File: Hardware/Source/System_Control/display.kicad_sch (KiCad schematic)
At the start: 9 parts, among them Q3 MMBT2222A, U5 LCD 5“SSD1963

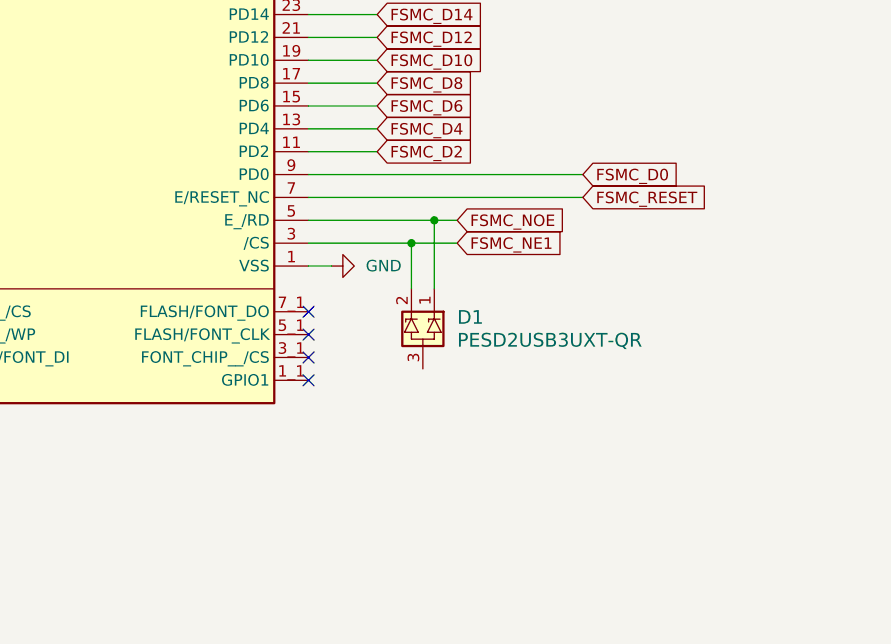
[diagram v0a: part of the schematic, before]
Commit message: update
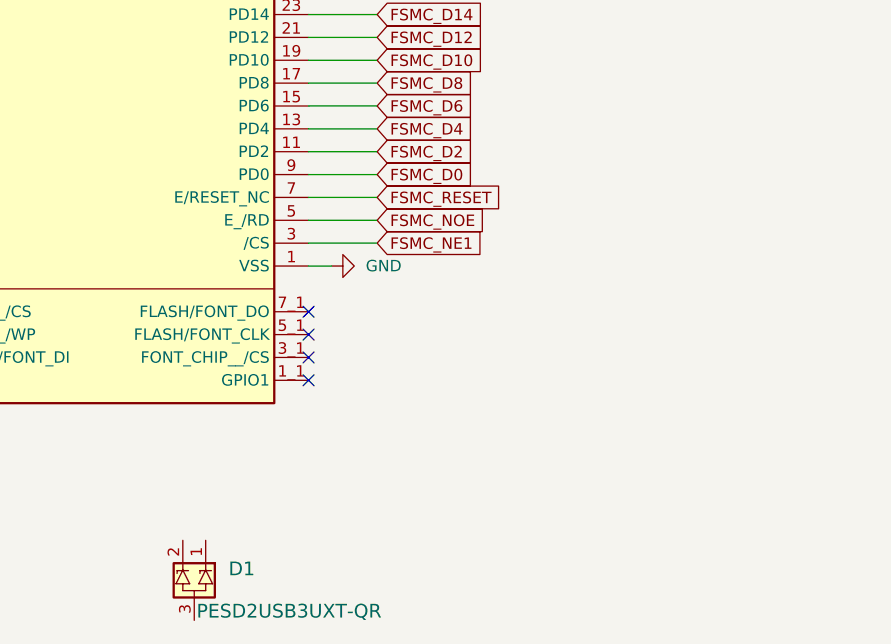
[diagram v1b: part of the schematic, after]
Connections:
- net FSMC_NE1: no longer D1.2
- net FSMC_NOE: no longer D1.1
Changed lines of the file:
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@@
 	(paper "A4")
-	(junction
-		(at 181.61 99.06)
-		(diameter 0)
-		(color 0 0 0 0)
-	)
 	(junction
 		(at 78.74 55.88)
@@
 	)
 	(junction
-		(at 179.07 101.6)
-		(diameter 0)
-		(color 0 0 0 0)
-	)
-	(junction
 		(at 241.3 100.33)
 		(diameter 0)
@@
 	(wire
 		(pts
-			(xy 179.07 101.6) (xy 167.64 101.6)
+			(xy 167.64 101.6) (xy 175.26 101.6)
 		)
 		(stroke
@@
 	(wire
 		(pts
-			(xy 184.15 99.06) (xy 181.61 99.06)
-		)
-		(stroke
-			(width 0)
-			(type default)
-		)
-	)
-	(wire
-		(pts
 			(xy 78.74 40.64) (xy 78.74 44.45)
 		)
@@
 	(wire
 		(pts
-			(xy 179.07 101.6) (xy 184.15 101.6)
-		)
-		(stroke
-			(width 0)
-			(type default)
-		)
-	)
-	(wire
-		(pts
 			(xy 115.57 63.5) (xy 123.19 63.5)
 		)
@@
 	(wire
 		(pts
-			(xy 198.12 93.98) (xy 167.64 93.98)
+			(xy 175.26 93.98) (xy 167.64 93.98)
 		)
 		(stroke
@@
 	(wire
 		(pts
-			(xy 167.64 96.52) (xy 198.12 96.52)
+			(xy 167.64 96.52) (xy 175.26 96.52)
 		)
 		(stroke
@@
 	(wire
 		(pts
-			(xy 181.61 99.06) (xy 167.64 99.06)
+			(xy 167.64 99.06) (xy 175.26 99.06)
 		)
 		(stroke
@@
 	(wire
 		(pts
-			(xy 179.07 101.6) (xy 179.07 106.68)
-		)
-		(stroke
-			(width 0)
-			(type default)
-		)
-	)
-	(wire
-		(pts
 			(xy 115.57 55.88) (xy 123.19 55.88)
 		)
@@
 		(pts
 			(xy 78.74 57.15) (xy 78.74 55.88)
-		)
-		(stroke
-			(width 0)
-			(type default)
-		)
-	)
-	(wire
-		(pts
-			(xy 181.61 99.06) (xy 181.61 106.68)
 		)
 		(stroke
@@
 	(global_label "FSMC_NE1"
 		(shape input)
-		(at 184.15 101.6 0)
+		(at 175.26 101.6 0)
 		(fields_autoplaced yes)
 		(effects
@@
 		)
 		(property "Intersheetrefs" "${INTERSHEET_REFS}"
-			(at 196.8113 101.6 0)
+			(at 187.9213 101.6 0)
 			(effects
 				(font
@@
 	(global_label "FSMC_NOE"
 		(shape input)
-		(at 184.15 99.06 0)
+		(at 175.26 99.06 0)
 		(fields_autoplaced yes)
 		(effects
@@
 		)
 		(property "Intersheetrefs" "${INTERSHEET_REFS}"
-			(at 196.9323 99.06 0)
+			(at 188.0423 99.06 0)
 			(effects
 				(font
@@
 	(global_label "FSMC_RESET"
 		(shape input)
-		(at 198.12 96.52 0)
+		(at 175.26 96.52 0)
 		(fields_autoplaced yes)
 		(effects
@@
 		)
 		(property "Intersheetrefs" "${INTERSHEET_REFS}"
-			(at 212.8374 96.52 0)
+			(at 189.9774 96.52 0)
 			(effects
 				(font
@@
 	(global_label "FSMC_D0"
 		(shape input)
-		(at 198.12 93.98 0)
+		(at 175.26 93.98 0)
 		(fields_autoplaced yes)
 		(effects
@@
 		)
 		(property "Intersheetrefs" "${INTERSHEET_REFS}"
-			(at 209.5718 93.98 0)
+			(at 186.7118 93.98 0)
 			(effects
 				(font
@@
 	)
 	(symbol
-		(lib_id "charge_battery_sym_lib:PESD2USB3UXT-QR")
-		(at 177.8 109.22 270)
-		(unit 1)
-		(exclude_from_sim no)
-		(in_bom yes)
-		(on_board yes)
-		(dnp no)
-		(fields_autoplaced yes)
-		(property "Reference" "D1"
-			(at 184.15 109.8549 90)
-			(effects
-				(font
-					(size 1.524 1.524)
-				)
-				(justify left)
-			)
-		)
-		(property "Value" "PESD2USB3UXT-QR"
-			(at 184.15 112.3949 90)
-			(effects
-				(font
-					(size 1.524 1.524)
-				)
-				(justify left)
-			)
-		)
-		(property "Footprint" "charge_battery_footprint_lib:SOT23"
-			(at 165.608 113.792 0)
-			(effects
-				(font
-					(size 1.27 1.27)
-					(italic yes)
-				)
-				(hide yes)
-			)
-		)
-		(property "Datasheet" "https://www.mouser.vn/datasheet/2/916/PESD2USB3UXT_Q-3435971.pdf"
-			(at 165.608 114.808 0)
-			(effects
-				(font
-					(size 1.27 1.27)
-					(italic yes)
-				)
-				(hide yes)
-			)
-		)
-		(property "Description" "ESD Protection Diodes / TVS Diodes SOT23 3.3V 4A AUTO ESD PROT"
-			(at 165.608 109.982 0)
-			(effects
-				(font
-					(size 1.27 1.27)
-				)
-				(hide yes)
-			)
-		)
-		(property "Supply name" "Mouser"
-			(at 165.608 110.49 0)
-			(effects
-				(font
-					(size 1.27 1.27)
-				)
-				(hide yes)
-			)
-		)
-		(property "Supply part number" "771-PESD2USB3UXT-QR"
-			(at 165.608 110.744 0)
-			(effects
-				(font
-					(size 1.27 1.27)
-				)
-				(hide yes)
-			)
-		)
-		(property "Supply URL" "https://www.mouser.vn/ProductDetail/Nexperia/PESD2USB3UXT-QR?qs=3Rah4i%252BhyCErbBl4ep9%252BDw%3D%3D"
-			(at 165.608 110.744 0)
-			(effects
-				(font
-					(size 1.27 1.27)
-				)
-				(hide yes)
-			)
-		)
-		(pin "3"
-		)
-		(pin "1"
-		)
-		(pin "2"
-		)
-		(instances
-			(project ""
-				(path "/85c53e8c-0403-413d-b6c5-0718d4365b1f/acaf0f73-9448-4a46-8e0c-1a18f2f42e7d"
-					(reference "D1")
-					(unit 1)
-				)
-			)
-		)
-	)
-	(symbol
 		(lib_id "charge_battery_sym_lib:Res_1K_0603_1%")
 		(at 39.37 62.23 0)
@@
 					(unit 1)
 				)
+			)
+		)
+	)
+	(symbol
+		(lib_id "charge_battery_sym_lib:PESD2USB3UXT-QR")
+		(at 152.4 137.16 270)
+		(unit 1)
+		(exclude_from_sim no)
+		(in_bom yes)
+		(on_board yes)
+		(dnp no)
+		(property "Reference" "D1"
+			(at 158.75 137.7949 90)
+			(effects
+				(font
+					(size 1.524 1.524)
+				)
+				(justify left)
+			)
+		)
+		(property "Value" "PESD2USB3UXT-QR"
+			(at 155.194 142.494 90)
+			(effects
+				(font
+					(size 1.524 1.524)
+				)
+				(justify left)
+			)
+		)
+		(property "Footprint" "charge_battery_footprint_lib:SOT23"
+			(at 140.208 141.732 0)
+			(effects
+				(font
+					(size 1.27 1.27)
+					(italic yes)
+				)
+				(hide yes)
+			)
+		)
+		(property "Datasheet" "https://www.mouser.vn/datasheet/2/916/PESD2USB3UXT_Q-3435971.pdf"
+			(at 140.208 142.748 0)
+			(effects
+				(font
+					(size 1.27 1.27)
+					(italic yes)
+				)
+				(hide yes)
+			)
+		)
+		(property "Description" "ESD Protection Diodes / TVS Diodes SOT23 3.3V 4A AUTO ESD PROT"
+			(at 140.208 137.922 0)
+			(effects
+				(font
+					(size 1.27 1.27)
+				)
+				(hide yes)
+			)
+		)
+		(property "Supply name" "Mouser"
+			(at 140.208 138.43 0)
+			(effects
+				(font
+					(size 1.27 1.27)
+				)
+				(hide yes)
+			)
+		)
+		(property "Supply part number" "771-PESD2USB3UXT-QR"
+			(at 140.208 138.684 0)
+			(effects
+				(font
+					(size 1.27 1.27)
+				)
+				(hide yes)
+			)
+		)
+		(property "Supply URL" "https://www.mouser.vn/ProductDetail/Nexperia/PESD2USB3UXT-QR?qs=3Rah4i%252BhyCErbBl4ep9%252BDw%3D%3D"
+			(at 140.208 138.684 0)
+			(effects
+				(font
+					(size 1.27 1.27)
+				)
+				(hide yes)
+			)
+		)
+		(pin "3"
+		)
+		(pin "1"
+		)
+		(pin "2"
+		)
+		(instances
+			(project "System_Control"
+				(path "/85c53e8c-0403-413d-b6c5-0718d4365b1f/acaf0f73-9448-4a46-8e0c-1a18f2f42e7d"
+					(reference "D1")
+					(unit 1)
+				)

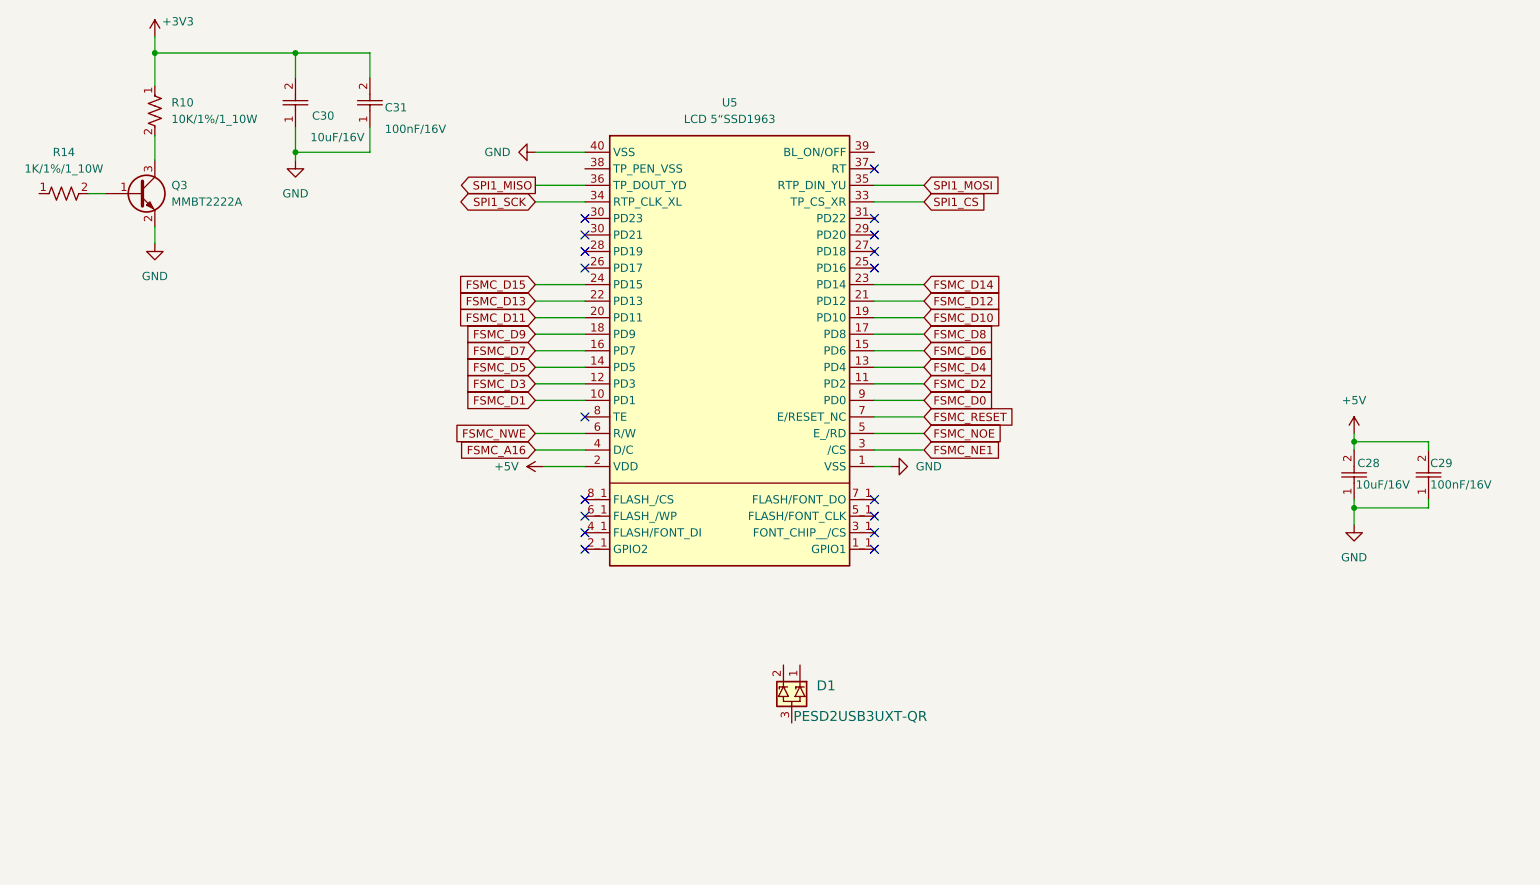
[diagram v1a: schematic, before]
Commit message: update footprint
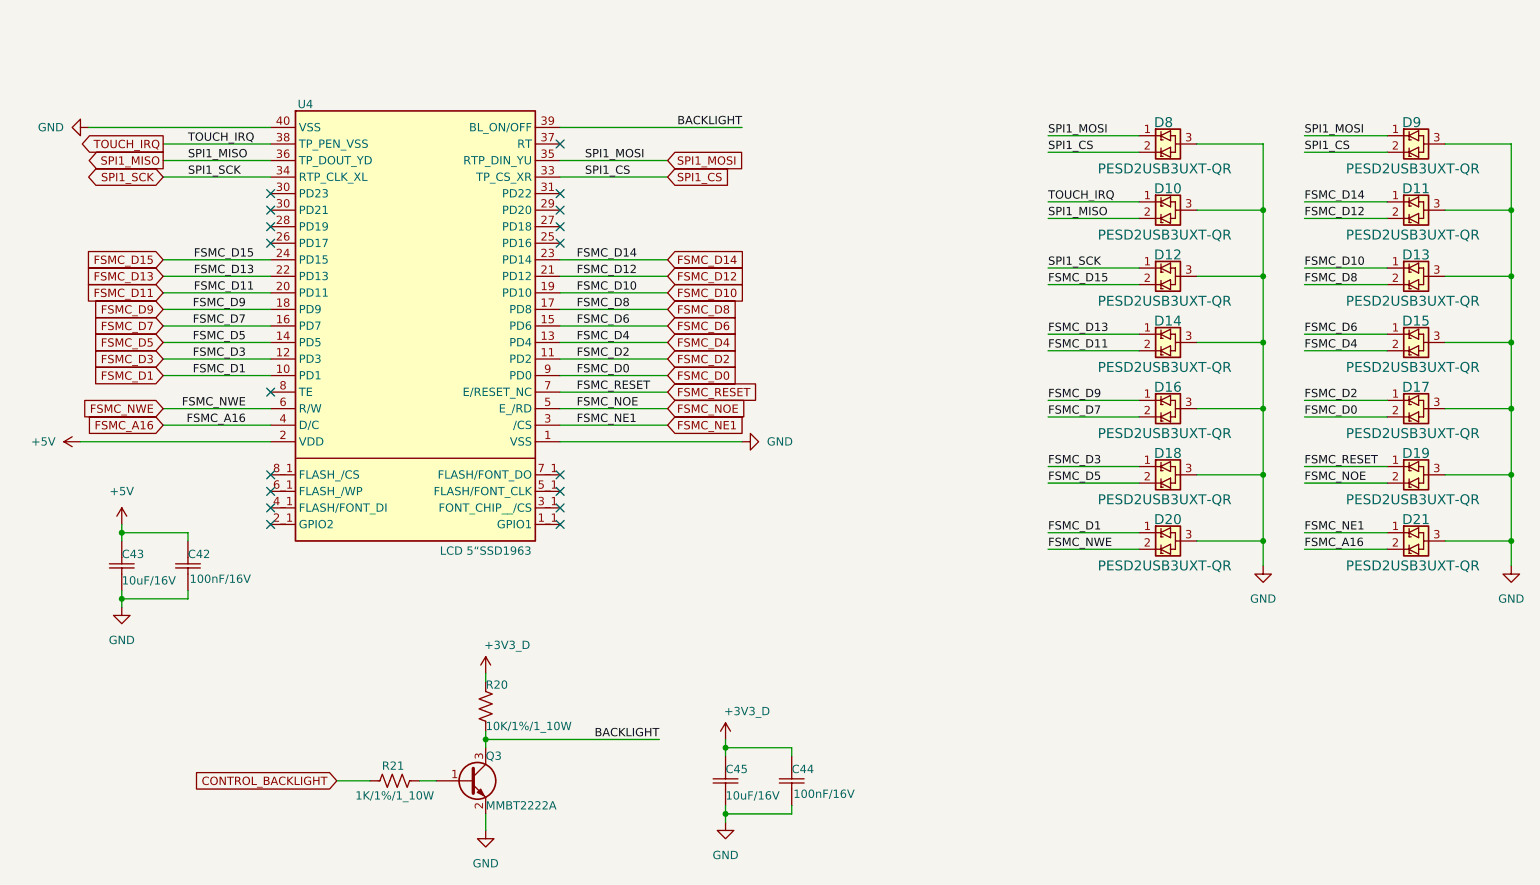
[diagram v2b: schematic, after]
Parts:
- removed C28, C30: 10uF/16V, charge_battery_footprint_lib:Ceramic_Cap_10uF_16V, symbol charge_battery_sym_lib:Ceramic_Cap_SMD_10uF_16V
- removed C29, C31: 100nF/16V, charge_battery_footprint_lib:C_0603_1608Metric, symbol charge_battery_sym_lib:Ceramic_Cap_SMD_100nF_16V
- removed R10: 10K/1%/1_10W, charge_battery_footprint_lib:Res_10K_0603, symbol charge_battery_sym_lib:Res_10K_0603_1%
- removed R14: 1K/1%/1_10W, charge_battery_footprint_lib:Res_1K_0603, symbol charge_battery_sym_lib:Res_1K_0603_1%
- added C42, C44: 100nF/16V, charge_battery_footprint_lib:Ceramic_Cap_0603, symbol charge_battery_sym_lib:Ceramic_Cap_SMD_100nF_16V
- added C43, C45: 10uF/16V, charge_battery_footprint_lib:Ceramic_Cap_0603, symbol charge_battery_sym_lib:Ceramic_Cap_SMD_10uF_16V
- added D10, D12, D13, D14, D15, D16, D17, D18, D19, D20, D21, D8, D9: PESD2USB3UXT-QR, charge_battery_footprint_lib:SOT23, symbol charge_battery_sym_lib:PESD2USB3UXT-QR
- added R20: 10K/1%/1_10W, charge_battery_footprint_lib:Res_0603, symbol charge_battery_sym_lib:Res_10K_0603_1%
- added R21: 1K/1%/1_10W, charge_battery_footprint_lib:Res_0603, symbol charge_battery_sym_lib:Res_1K_0603_1%
- U4: renamed from U5; footprint (none) -> charge_battery_footprint_lib:LCD 5“SSD1963 TFT Module
- renumbered D1 to D11
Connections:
- net +5V: now also C42.2, C43.2
- net FSMC_A16: now also D21.2
- net FSMC_D0: now also D17.2
- net FSMC_D1: now also D20.1
- net FSMC_D10: now also D13.1
- net FSMC_D11: now also D14.2
- net FSMC_D12: now also D11.2
- net FSMC_D13: now also D14.1
- net FSMC_D14: now also D11.1
- net FSMC_D15: now also D12.2
- net FSMC_D2: now also D17.1
- net FSMC_D3: now also D18.1
- net FSMC_D4: now also D15.2
- net FSMC_D5: now also D18.2
- net FSMC_D6: now also D15.1
- net FSMC_D7: now also D16.2
- net FSMC_D8: now also D13.2
- net FSMC_D9: now also D16.1
- net FSMC_NE1: now also D21.1
- net FSMC_NOE: now also D19.2
- net FSMC_NWE: now also D20.2
- net FSMC_RESET: now also D19.1
- net GND: now also D11.3, C42.1, C43.1, C44.1, C45.1, D10.3, D12.3, D13.3, D14.3, D15.3, D16.3, D17.3, D18.3, D19.3, D20.3, D21.3, D8.3, D9.3
- net SPI1_CS: now also D8.2, D9.2
- net SPI1_MISO: now also D10.2
- net SPI1_MOSI: now also D8.1, D9.1
- net SPI1_SCK: now also D12.1
- net at Q3.1 (B): now also R21.2
- net BACKLIGHT: now reaches Q3.3 (C)
- net BACKLIGHT: now also U4.39 (BL_ON/OFF), R20.1
- net TOUCH_IRQ: now reaches U4.38 (TP_PEN_VSS)
- net TOUCH_IRQ: now also D10.1
- new net +3V3_D: C44.2, C45.2, R20.2
- new net CONTROL_BACKLIGHT: R21.1
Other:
- moved on the sheet: D11, Q3, U4
